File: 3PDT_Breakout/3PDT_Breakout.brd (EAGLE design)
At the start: 33.5 x 24.4 mm, 12 parts

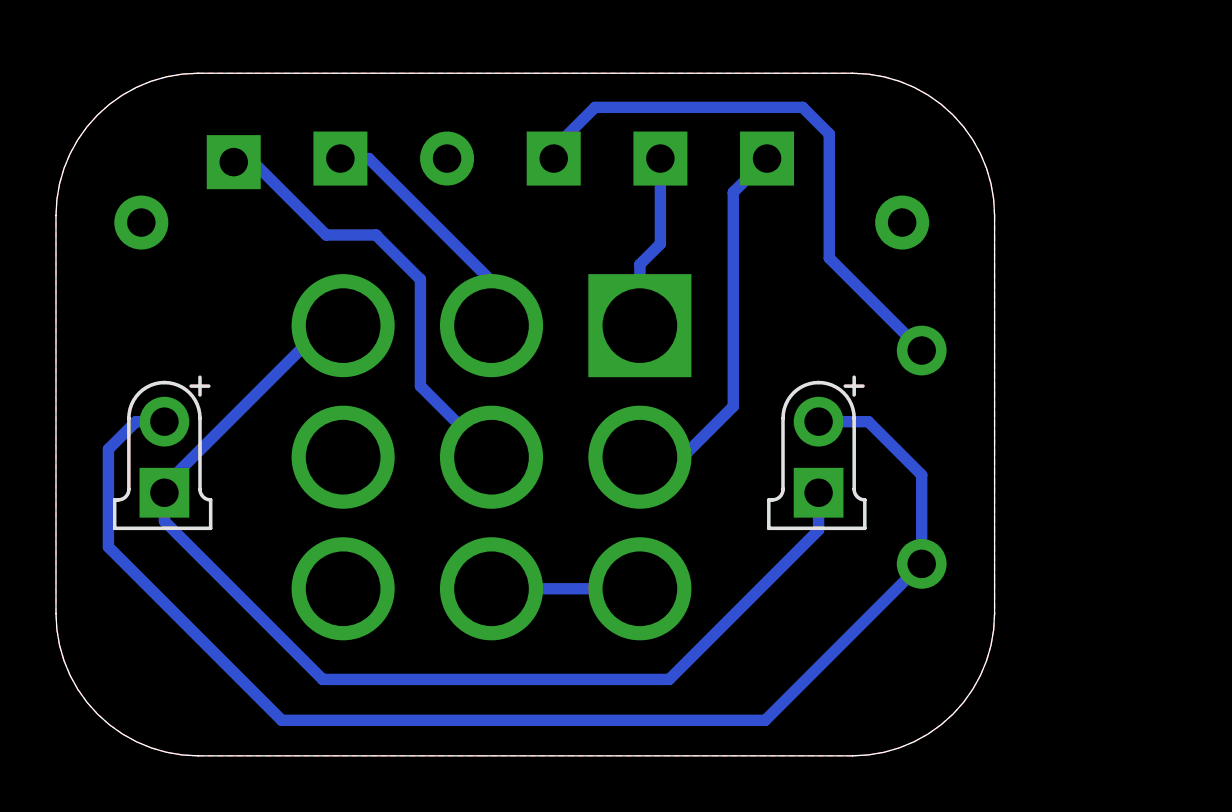
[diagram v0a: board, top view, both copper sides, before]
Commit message: Added boards
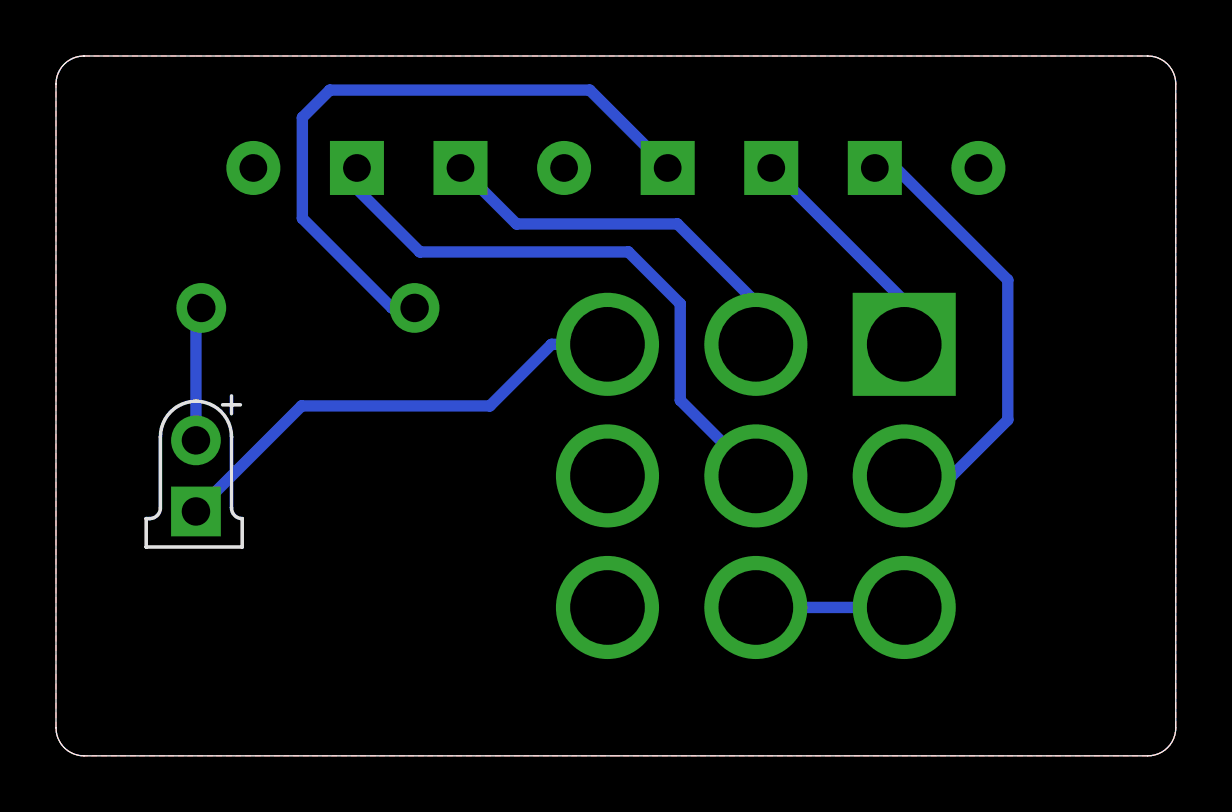
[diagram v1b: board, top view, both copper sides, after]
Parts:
- removed CI, CO: PADS.SQR_NL, supply pins:PAD4
- removed GI, GND, GO: GND_PADROUND, supply pins:ROUND
- removed I: IN, supply pins:SQUARE
- removed LED: LED3MM, diodes:LED3MM
- removed O: OUT, supply pins:SQUARE
- removed V+: +9V_PAD, supply pins:SQUARE
- added U$1: HEADERS8, my_headers:HEADERS8
- moved CLR 22.6 mm to (9.00, 16.0), turned to 180 degrees
- moved 3PDT 9.47 mm to (25.0, 10.0)
- moved LED1 1.31 mm to (5.00, 10.0)
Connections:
- removed net N$3: 3PDT.B1, CO.P$1
- removed net N$4: 3PDT.A1, CI.P$1
- new net CI: 3PDT.B1, U$1.CI
- new net CO: 3PDT.A1, U$1.CO
- net +9V: now also U$1.+9V; no longer V+.1
- net GND: now also U$1.G1, U$1.G2, U$1.GND; no longer GI.1, GND.1, GO.1
- net IN: now also 3PDT.B2, U$1.IN; no longer 3PDT.A2, I.1
- net N$1: no longer LED.K
- net N$2: no longer LED.A
- net OUT: now also 3PDT.A2, U$1.OUT; no longer 3PDT.B2, O.1
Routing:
- net N$2: track 47.5 -> 4.81 mm
- net N$1: track 39.3 -> 17.2 mm
- net CI: track 0.00 -> 14.0 mm
- net N$3: track 8.80 -> 0.00 mm
- net CO: track 0.00 -> 8.27 mm
- net IN: track 13.4 -> 21.3 mm
- net N$4: track 6.27 -> 0.00 mm
- net +9V: track 20.3 -> 23.5 mm
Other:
- board size 33.5 x 24.4 mm -> 40 x 25 mm
- board text added: "REV 0.0"
- board text removed: "CI"
- board text removed: "CO"
